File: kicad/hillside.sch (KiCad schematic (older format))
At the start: 83 parts, among them J1 Haptic, J2 TRRS, J3 Bat_Pos, J4 Bat_GND, K1 SW_Key, K10 SW_Key, K11 SW_Key, K12 SW_Key, K13 SW_Key, K14 SW_Key, K15 SW_Key, K16 SW_Key, K17 SW_Key, K18 SW_Key, K19 SW_Key, K2 SW_Key, K20 SW_Rotary, K21 SW_Key, K22 SW_Key, K23 SW_Key, K24 SW_Key, K3 SW_Key, K4 SW_Key, K5 SW_Key, K6 SW_Key, K7 SW_Key, K8 SW_Key, K9 SW_Key, SW1 Reset, SW2 SW_Power, U1 ProMicro_r

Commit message: Sym/Footprint: rename logo, cleanups
- remove unused choc-diode sym
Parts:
- H3: value Scene -> Logo; footprint hillside:Hillside_Scene -> hillside:Hillside_Logo; symbol hillside:Scene -> hillside:Logo
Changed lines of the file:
@@
 NoConn ~ 9100 1650
 $Comp
-L hillside:Scene H3
+L hillside:Logo H3
 U 1 1 62029C5C
 P 850 7050
 F 0 "H3" H 1100 7200 50  0000 L CNN
-F 1 "Scene" H 1100 7100 50  0000 L CNN
-F 2 "hillside:Hillside_Scene" H 850 6800 50  0001 C CNN
+F 1 "Logo" H 1100 7100 50  0000 L CNN
+F 2 "hillside:Hillside_Logo" H 850 6800 50  0001 C CNN
 F 3 "" H 850 6800 50  0001 C CNN
 	1    850  7050

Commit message: Common symbols/footprints used in hillside_basic
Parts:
- C1: footprint ki_syms:C_0805_2012Metric -> hillside_basic:C_0805_2012Metric; symbol ki_syms:C -> hillside_basic:C
- D1, D2, D3, D4, D5: footprint ki_syms:SK6812-MINI-E -> hillside_basic:SK6812-MINI-E; symbol ki_syms:SK6812-MINI-E -> hillside_basic:SK6812-MINI-E
- D10, D11, D12, D13, D14, D15, D16, D17, D18, D7, D8, D9: footprint ki_syms:SOT-23 -> hillside_basic:SOT-23; symbol ki_syms:BAV70_Small -> hillside_basic:BAV70_Small
- H4, H5, H8, H9: footprint ki_syms:MountingHole_2.2mm_M2_Pad -> hillside_basic:MountingHole_2.2mm_M2_Pad; symbol ki_mech:MountingHole -> hillside_basic:MountingHole
- H6, H7: footprint ki_syms:MountingHole_2.2mm_M2 -> hillside_basic:MountingHole_2.2mm_M2; symbol ki_mech:MountingHole -> hillside_basic:MountingHole
- J1: symbol ki_syms:Conn_01x05-Connector_Generic -> hillside_basic:Conn_01x05-Connector_Generic
- J3, J4: footprint ki_syms:1pin_conn -> hillside_basic:1pin_conn; symbol ki_conn_generic:Conn_01x01 -> hillside_basic:Conn_01x01
- JP1: footprint ki_syms:SolderJumper-2_P1.3mm_Bridged_RoundedPad1.0x1.5mm -> hillside_basic:SolderJumper-2_P1.3mm_Bridged_RoundedPad1.0x1.5mm; symbol ki_jumper:SolderJumper_2_Bridged -> hillside_basic:SolderJumper_2_Bridged
- R1, R2: footprint ki_syms:R_0805_2012Metric -> hillside_basic:R_0805_2012Metric; symbol ki_syms:R -> hillside_basic:R
- SW1: footprint ki_syms:SW_SPST_SKQG_WithStem -> hillside_basic:SW_SPST_SKQG_WithStem
- SW2: footprint ki_syms:SW_SPDT_JS202011AQN -> hillside_basic:SW_SPDT_JS202011AQN; symbol ki_switch:SW_SPDT -> hillside_basic:SW_SPDT
- V1, V10, V11, V12, V13, V14, V15, V16, V17, V18, V19, V2, V20, V21, V22, V3, V4, V5, V6, V7, V8, V9: footprint ki_syms:VIA-0.8mm -> hillside_basic:VIA-0.8mm; symbol ki_syms:Via -> hillside_basic:Via

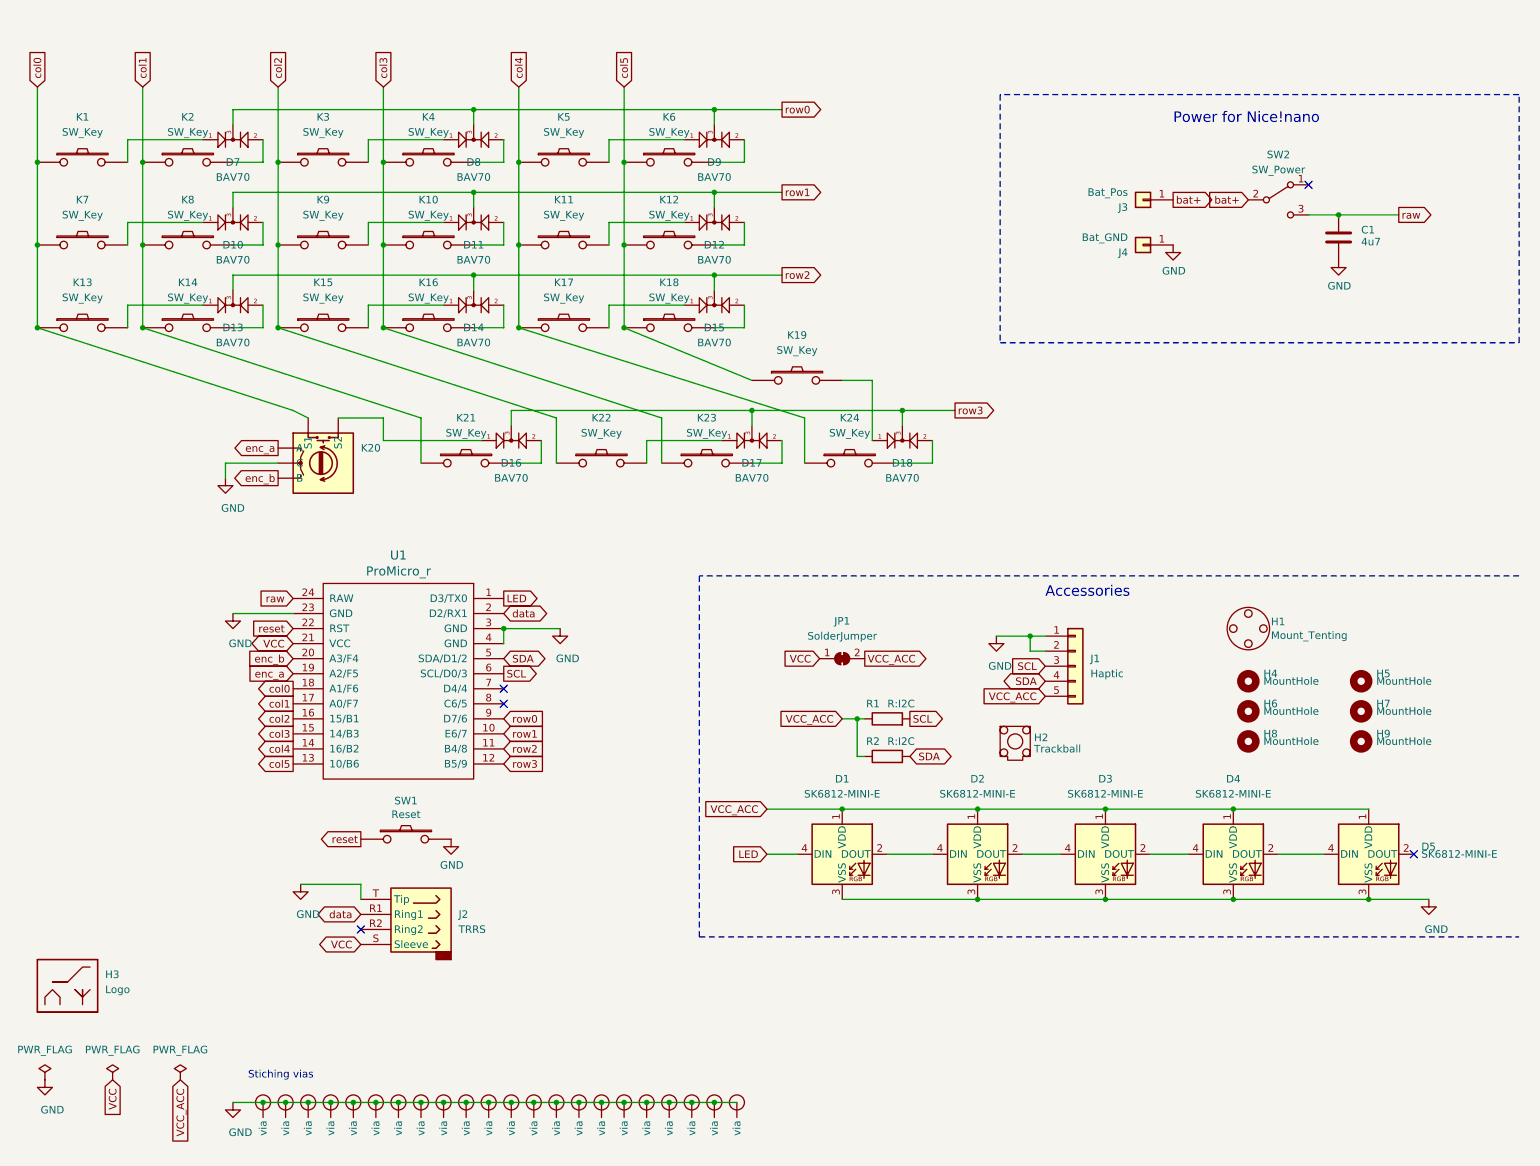
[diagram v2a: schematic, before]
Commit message: - cleanup schema sheet
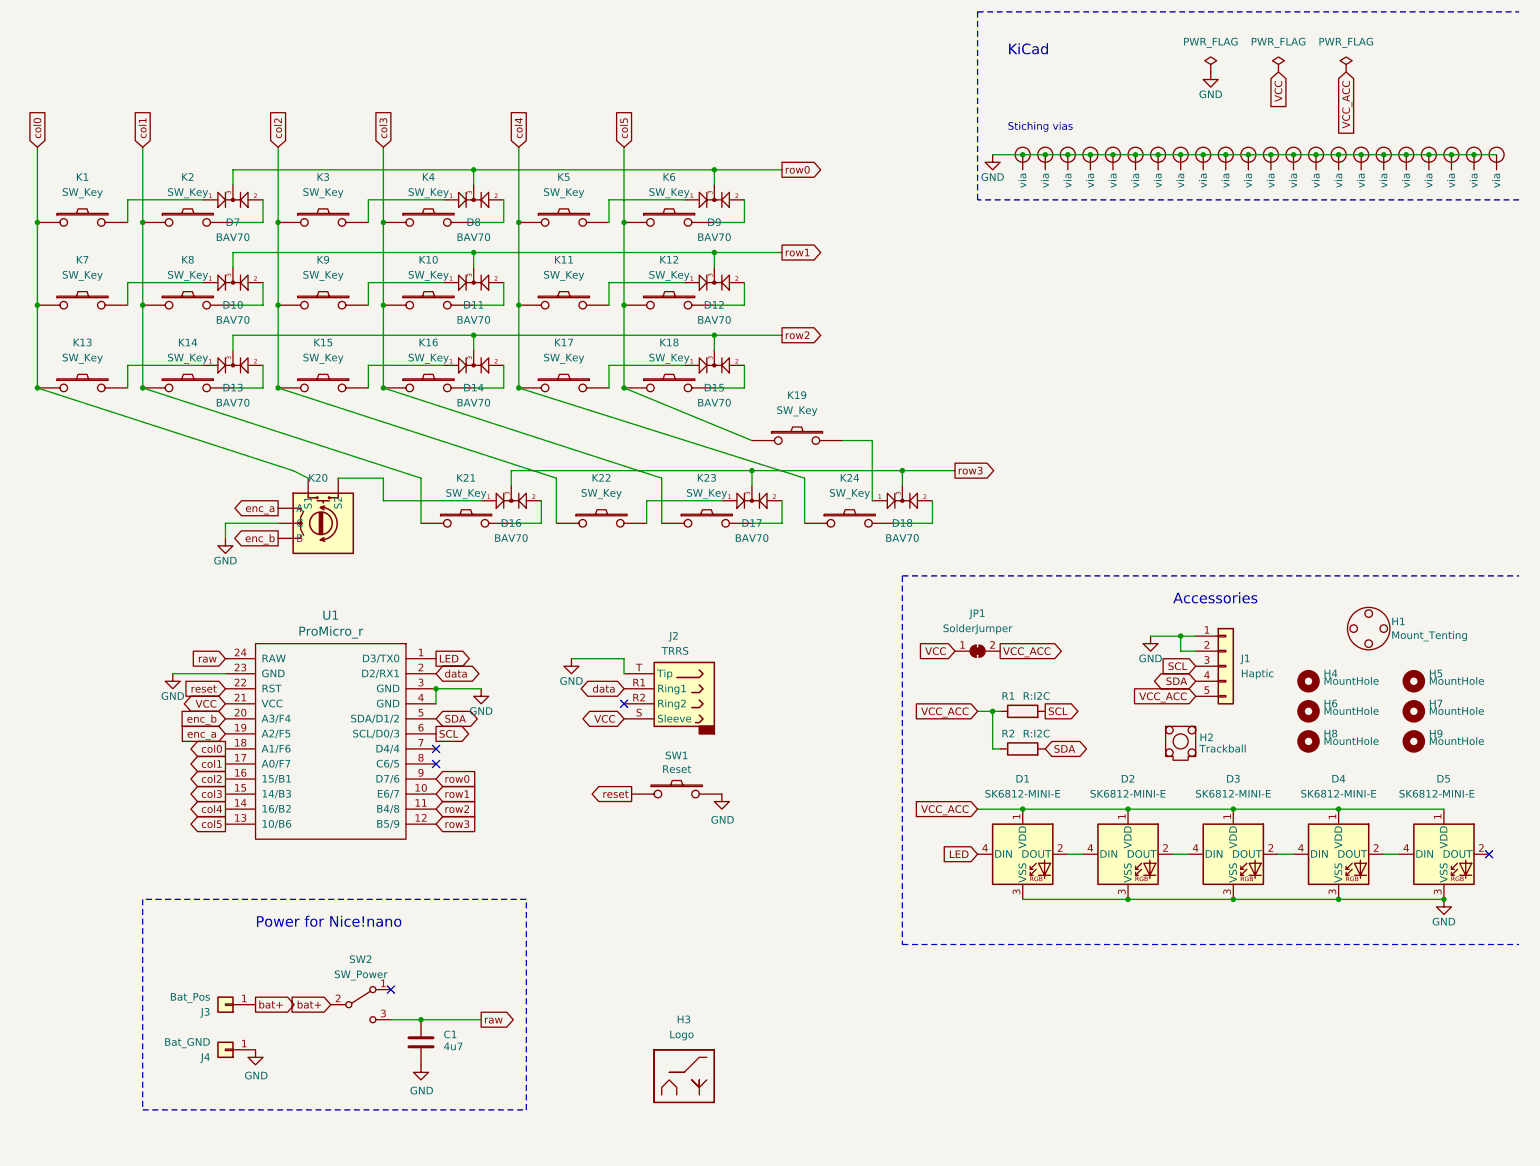
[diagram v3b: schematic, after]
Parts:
- V1: value V -> Via
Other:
- note added: "KiCad"
- moved on the sheet: C1, D1, D10, D11, D12, D13, D14, D15, D16, D17, D18, D2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
